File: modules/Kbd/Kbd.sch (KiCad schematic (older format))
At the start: 43 parts, among them J1 2, J10 11, J11 12, J12 13, J13 A0, J14 A1, J15 A2, J16 A3, J17 A4, J18 A5, J19 Vcc, J2 3, J20 Gnd, J3 4, J4 5, J5 6, J6 7, J7 8, J8 9, J9 10

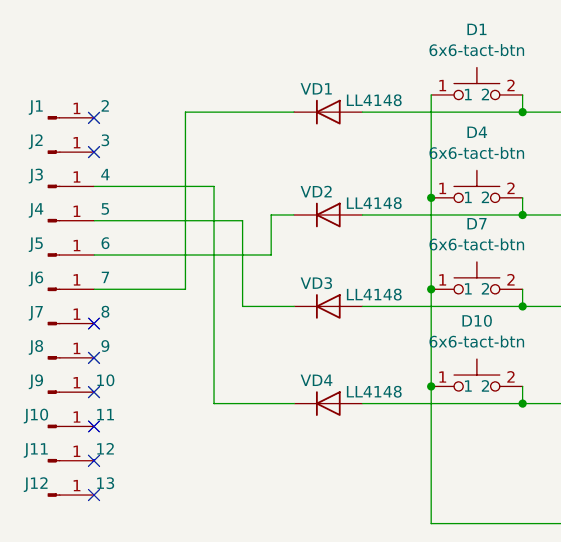
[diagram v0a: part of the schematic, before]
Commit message: Kbd v2. Fixed pin numbering.
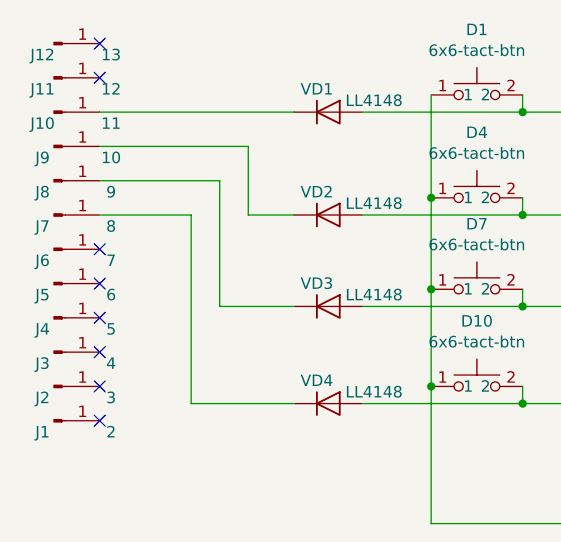
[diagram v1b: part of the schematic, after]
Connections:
- net at J3.1 (Pin_1): no longer VD4.1 (K)
- net at J4.1 (Pin_1): no longer VD3.1 (K)
- net at J5.1 (Pin_1): no longer VD2.1 (K)
- net at J6.1 (Pin_1): no longer VD1.1 (K)
- net at J7.1 (Pin_1): now also VD4.1 (K)
- net at J8.1 (Pin_1): now also VD3.1 (K)
- net at J9.1 (Pin_1): now also VD2.1 (K)
- net at J10.1 (Pin_1): now also VD1.1 (K)
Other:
- moved on the sheet: J1, J10, J11, J12, J2, J3, J4, J5, J6, J7, J8, J9
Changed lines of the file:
@@
 EESchema Schematic File Version 4
-LIBS:Kbd-cache
 EELAYER 30 0
 EELAYER END
@@
 L Connector:Conn_01x01_Male J1
 U 1 1 5D793457
-P 1025 2500
-F 0 "J1" H 975 2550 50  0000 C CNN
-F 1 "2" H 1275 2550 50  0000 C CNN
-F 2 "Connector_PinHeader_2.54mm:PinHeader_1x01_P2.54mm_Vertical" H 1025 2500 50  0001 C CNN
-F 3 "~" H 1025 2500 50  0001 C CNN
-	1    1025 2500
-	1    0    0    -1
+P 1050 3825
+F 0 "J1" H 1000 3875 50  0000 C CNN
+F 1 "2" H 1300 3875 50  0000 C CNN
+F 2 "Connector_PinHeader_2.54mm:PinHeader_1x01_P2.54mm_Vertical" H 1050 3825 50  0001 C CNN
+F 3 "~" H 1050 3825 50  0001 C CNN
+	1    1050 3825
+	1    0    0    1
 $EndComp
 $Comp
 L Connector:Conn_01x01_Male J2
 U 1 1 5D794940
-P 1025 2650
-F 0 "J2" H 975 2700 50  0000 C CNN
-F 1 "3" H 1275 2700 50  0000 C CNN
-F 2 "Connector_PinHeader_2.54mm:PinHeader_1x01_P2.54mm_Vertical" H 1025 2650 50  0001 C CNN
-F 3 "~" H 1025 2650 50  0001 C CNN
-	1    1025 2650
-	1    0    0    -1
+P 1050 3675
+F 0 "J2" H 1000 3725 50  0000 C CNN
+F 1 "3" H 1300 3725 50  0000 C CNN
+F 2 "Connector_PinHeader_2.54mm:PinHeader_1x01_P2.54mm_Vertical" H 1050 3675 50  0001 C CNN
+F 3 "~" H 1050 3675 50  0001 C CNN
+	1    1050 3675
+	1    0    0    1
 $EndComp
 $Comp
 L Connector:Conn_01x01_Male J3
 U 1 1 5D794B32
-P 1025 2800
-F 0 "J3" H 975 2850 50  0000 C CNN
-F 1 "4" H 1275 2850 50  0000 C CNN
-F 2 "Connector_PinHeader_2.54mm:PinHeader_1x01_P2.54mm_Vertical" H 1025 2800 50  0001 C CNN
-F 3 "~" H 1025 2800 50  0001 C CNN
-	1    1025 2800
-	1    0    0    -1
-$EndComp
-$Comp
-L Connector:Conn_01x01_Male J4
-U 1 1 5D794C66
-P 1025 2950
-F 0 "J4" H 975 3000 50  0000 C CNN
-F 1 "5" H 1275 3000 50  0000 C CNN
-F 2 "Connector_PinHeader_2.54mm:PinHeader_1x01_P2.54mm_Vertical" H 1025 2950 50  0001 C CNN
-F 3 "~" H 1025 2950 50  0001 C CNN
-	1    1025 2950
-	1    0    0    -1
+P 1050 3525
+F 0 "J3" H 1000 3575 50  0000 C CNN
+F 1 "4" H 1300 3575 50  0000 C CNN
+F 2 "Connector_PinHeader_2.54mm:PinHeader_1x01_P2.54mm_Vertical" H 1050 3525 50  0001 C CNN
+F 3 "~" H 1050 3525 50  0001 C CNN
+	1    1050 3525
+	1    0    0    1
 $EndComp
 $Comp
 L Connector:Conn_01x01_Male J5
 U 1 1 5D794EF4
-P 1025 3100
-F 0 "J5" H 975 3150 50  0000 C CNN
-F 1 "6" H 1275 3150 50  0000 C CNN
-F 2 "Connector_PinHeader_2.54mm:PinHeader_1x01_P2.54mm_Vertical" H 1025 3100 50  0001 C CNN
-F 3 "~" H 1025 3100 50  0001 C CNN
-	1    1025 3100
-	1    0    0    -1
+P 1050 3225
+F 0 "J5" H 1000 3275 50  0000 C CNN
+F 1 "6" H 1300 3275 50  0000 C CNN
+F 2 "Connector_PinHeader_2.54mm:PinHeader_1x01_P2.54mm_Vertical" H 1050 3225 50  0001 C CNN
+F 3 "~" H 1050 3225 50  0001 C CNN
+	1    1050 3225
+	1    0    0    1
 $EndComp
 $Comp
 L Connector:Conn_01x01_Male J6
 U 1 1 5D795168
-P 1025 3250
-F 0 "J6" H 975 3300 50  0000 C CNN
-F 1 "7" H 1275 3300 50  0000 C CNN
-F 2 "Connector_PinHeader_2.54mm:PinHeader_1x01_P2.54mm_Vertical" H 1025 3250 50  0001 C CNN
-F 3 "~" H 1025 3250 50  0001 C CNN
-	1    1025 3250
-	1    0    0    -1
+P 1050 3075
+F 0 "J6" H 1000 3125 50  0000 C CNN
+F 1 "7" H 1300 3125 50  0000 C CNN
+F 2 "Connector_PinHeader_2.54mm:PinHeader_1x01_P2.54mm_Vertical" H 1050 3075 50  0001 C CNN
+F 3 "~" H 1050 3075 50  0001 C CNN
+	1    1050 3075
+	1    0    0    1
 $EndComp
 $Comp
 L Connector:Conn_01x01_Male J7
 U 1 1 5D795340
-P 1025 3400
-F 0 "J7" H 975 3450 50  0000 C CNN
-F 1 "8" H 1275 3450 50  0000 C CNN
-F 2 "Connector_PinHeader_2.54mm:PinHeader_1x01_P2.54mm_Vertical" H 1025 3400 50  0001 C CNN
-F 3 "~" H 1025 3400 50  0001 C CNN
-	1    1025 3400
-	1    0    0    -1
+P 1050 2925
+F 0 "J7" H 1000 2975 50  0000 C CNN
+F 1 "8" H 1300 2975 50  0000 C CNN
+F 2 "Connector_PinHeader_2.54mm:PinHeader_1x01_P2.54mm_Vertical" H 1050 2925 50  0001 C CNN
+F 3 "~" H 1050 2925 50  0001 C CNN
+	1    1050 2925
+	1    0    0    1
 $EndComp
 $Comp
 L Connector:Conn_01x01_Male J8
 U 1 1 5D7955DE
-P 1025 3550
-F 0 "J8" H 975 3600 50  0000 C CNN
-F 1 "9" H 1275 3600 50  0000 C CNN
-F 2 "Connector_PinHeader_2.54mm:PinHeader_1x01_P2.54mm_Vertical" H 1025 3550 50  0001 C CNN
-F 3 "~" H 1025 3550 50  0001 C CNN
-	1    1025 3550
-	1    0    0    -1
+P 1050 2775
+F 0 "J8" H 1000 2825 50  0000 C CNN
+F 1 "9" H 1300 2825 50  0000 C CNN
+F 2 "Connector_PinHeader_2.54mm:PinHeader_1x01_P2.54mm_Vertical" H 1050 2775 50  0001 C CNN
+F 3 "~" H 1050 2775 50  0001 C CNN
+	1    1050 2775
+	1    0    0    1
 $EndComp
 $Comp
 L Connector:Conn_01x01_Male J9
 U 1 1 5D7957DA
-P 1025 3700
-F 0 "J9" H 975 3750 50  0000 C CNN
-F 1 "10" H 1275 3750 50  0000 C CNN
-F 2 "Connector_PinHeader_2.54mm:PinHeader_1x01_P2.54mm_Vertical" H 1025 3700 50  0001 C CNN
-F 3 "~" H 1025 3700 50  0001 C CNN
-	1    1025 3700
-	1    0    0    -1
+P 1050 2625
+F 0 "J9" H 1000 2675 50  0000 C CNN
+F 1 "10" H 1300 2675 50  0000 C CNN
+F 2 "Connector_PinHeader_2.54mm:PinHeader_1x01_P2.54mm_Vertical" H 1050 2625 50  0001 C CNN
+F 3 "~" H 1050 2625 50  0001 C CNN
+	1    1050 2625
+	1    0    0    1
 $EndComp
 $Comp
 L Connector:Conn_01x01_Male J10
 U 1 1 5D795810
-P 1025 3850
-F 0 "J10" H 975 3900 50  0000 C CNN
-F 1 "11" H 1275 3900 50  0000 C CNN
-F 2 "Connector_PinHeader_2.54mm:PinHeader_1x01_P2.54mm_Vertical" H 1025 3850 50  0001 C CNN
-F 3 "~" H 1025 3850 50  0001 C CNN
-	1    1025 3850
-	1    0    0    -1
+P 1050 2475
+F 0 "J10" H 1000 2525 50  0000 C CNN
+F 1 "11" H 1300 2525 50  0000 C CNN
+F 2 "Connector_PinHeader_2.54mm:PinHeader_1x01_P2.54mm_Vertical" H 1050 2475 50  0001 C CNN
+F 3 "~" H 1050 2475 50  0001 C CNN
+	1    1050 2475
+	1    0    0    1
 $EndComp
 $Comp
 L Connector:Conn_01x01_Male J11
 U 1 1 5D7959D6
-P 1025 4000
-F 0 "J11" H 975 4050 50  0000 C CNN
-F 1 "12" H 1275 4050 50  0000 C CNN
-F 2 "Connector_PinHeader_2.54mm:PinHeader_1x01_P2.54mm_Vertical" H 1025 4000 50  0001 C CNN
-F 3 "~" H 1025 4000 50  0001 C CNN
-	1    1025 4000
-	1    0    0    -1
+P 1050 2325
+F 0 "J11" H 1000 2375 50  0000 C CNN
+F 1 "12" H 1300 2375 50  0000 C CNN
+F 2 "Connector_PinHeader_2.54mm:PinHeader_1x01_P2.54mm_Vertical" H 1050 2325 50  0001 C CNN
+F 3 "~" H 1050 2325 50  0001 C CNN
+	1    1050 2325
+	1    0    0    1
 $EndComp
 $Comp
@@
 L Connector:Conn_01x01_Male J12
 U 1 1 5D79744D
-P 1025 4150
-F 0 "J12" H 975 4200 50  0000 C CNN
-F 1 "13" H 1275 4200 50  0000 C CNN
-F 2 "Connector_PinHeader_2.54mm:PinHeader_1x01_P2.54mm_Vertical" H 1025 4150 50  0001 C CNN
-F 3 "~" H 1025 4150 50  0001 C CNN
-	1    1025 4150
-	1    0    0    -1
+P 1050 2175
+F 0 "J12" H 1000 2225 50  0000 C CNN
+F 1 "13" H 1300 2225 50  0000 C CNN
+F 2 "Connector_PinHeader_2.54mm:PinHeader_1x01_P2.54mm_Vertical" H 1050 2175 50  0001 C CNN
+F 3 "~" H 1050 2175 50  0001 C CNN
+	1    1050 2175
+	1    0    0    1
 $EndComp
 $Comp
@@
 	6000 2800 6750 2800
 Connection ~ 2700 3675
-$Comp
-L Diode:LL4148 VD1
-U 1 1 5E4DB037
-P 2250 2475
-F 0 "VD1" H 2200 2575 50  0000 C CNN
-F 1 "LL4148" H 2450 2525 50  0000 C CNN
-F 2 "Diode_SMD:D_MiniMELF" H 2250 2300 50  0001 C CNN
-F 3 "http://www.vishay.com/docs/85557/ll4148.pdf" H 2250 2475 50  0001 C CNN
-	1    2250 2475
-	1    0    0    -1
-$EndComp
 $Comp
 L Diode:LL4148 VD2
@@
 Wire Wire Line
 	6750 3550 6425 3550
-NoConn ~ 1225 2500
-NoConn ~ 1225 2650
-NoConn ~ 1225 3400
-NoConn ~ 1225 3550
-NoConn ~ 1225 3700
-NoConn ~ 1225 3850
-NoConn ~ 1225 4000
-NoConn ~ 1225 4150
+NoConn ~ 1250 3825
+NoConn ~ 1250 3675
+NoConn ~ 1250 3075
+NoConn ~ 1250 3225
+NoConn ~ 1250 3375
+NoConn ~ 1250 3525
+NoConn ~ 1250 2325
+NoConn ~ 1250 2175
 NoConn ~ 6750 2950
 NoConn ~ 6750 3100
@@
 	2400 3750 3100 3750
 Connection ~ 3100 3750
-Wire Wire Line
-	1750 2800 1750 3750
-Wire Wire Line
-	1750 3750 2100 3750
-Wire Wire Line
-	1225 2800 1750 2800
-Wire Wire Line
-	1225 2950 1875 2950
-Wire Wire Line
-	1875 2950 1875 3325
-Wire Wire Line
-	1875 3325 2100 3325
-Wire Wire Line
-	2000 3100 2000 2925
-Wire Wire Line
-	2000 2925 2100 2925
-Wire Wire Line
-	1225 3100 2000 3100
-Wire Wire Line
-	1225 3250 1625 3250
-Wire Wire Line
-	1625 3250 1625 2475
-Wire Wire Line
-	1625 2475 2100 2475
+$Comp
+L Connector:Conn_01x01_Male J4
+U 1 1 5D794C66
+P 1050 3375
+F 0 "J4" H 1000 3425 50  0000 C CNN
+F 1 "5" H 1300 3425 50  0000 C CNN
+F 2 "Connector_PinHeader_2.54mm:PinHeader_1x01_P2.54mm_Vertical" H 1050 3375 50  0001 C CNN
+F 3 "~" H 1050 3375 50  0001 C CNN
+	1    1050 3375
+	1    0    0    1
+$EndComp
+$Comp
+L Diode:LL4148 VD1
+U 1 1 5E4DB037
+P 2250 2475
+F 0 "VD1" H 2200 2575 50  0000 C CNN
+F 1 "LL4148" H 2450 2525 50  0000 C CNN
+F 2 "Diode_SMD:D_MiniMELF" H 2250 2300 50  0001 C CNN
+F 3 "http://www.vishay.com/docs/85557/ll4148.pdf" H 2250 2475 50  0001 C CNN
+	1    2250 2475
+	1    0    0    -1
+$EndComp
+Wire Wire Line
+	1250 2475 2100 2475
+Wire Wire Line
+	1250 2625 1900 2625
+Wire Wire Line
+	1900 2625 1900 2925
+Wire Wire Line
+	1900 2925 2100 2925
+Wire Wire Line
+	1250 2775 1775 2775
+Wire Wire Line
+	1775 2775 1775 3325
+Wire Wire Line
+	1775 3325 2100 3325
+Wire Wire Line
+	1250 2925 1650 2925
+Wire Wire Line
+	1650 2925 1650 3750
+Wire Wire Line
+	1650 3750 2100 3750
 $EndSCHEMATC
